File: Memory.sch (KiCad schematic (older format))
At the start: 18 parts, among them U10 74LS05, U11 74HCT00, U12 74LS32, U2 AS6C4008-55PCN, U3 AS6C4008-55PCN, U4 AS6C4008-55PCN, U5 AS6C4008-55PCN, U6 74HCT00, U7 74LS32, U8 74LS32, U9 74LS05

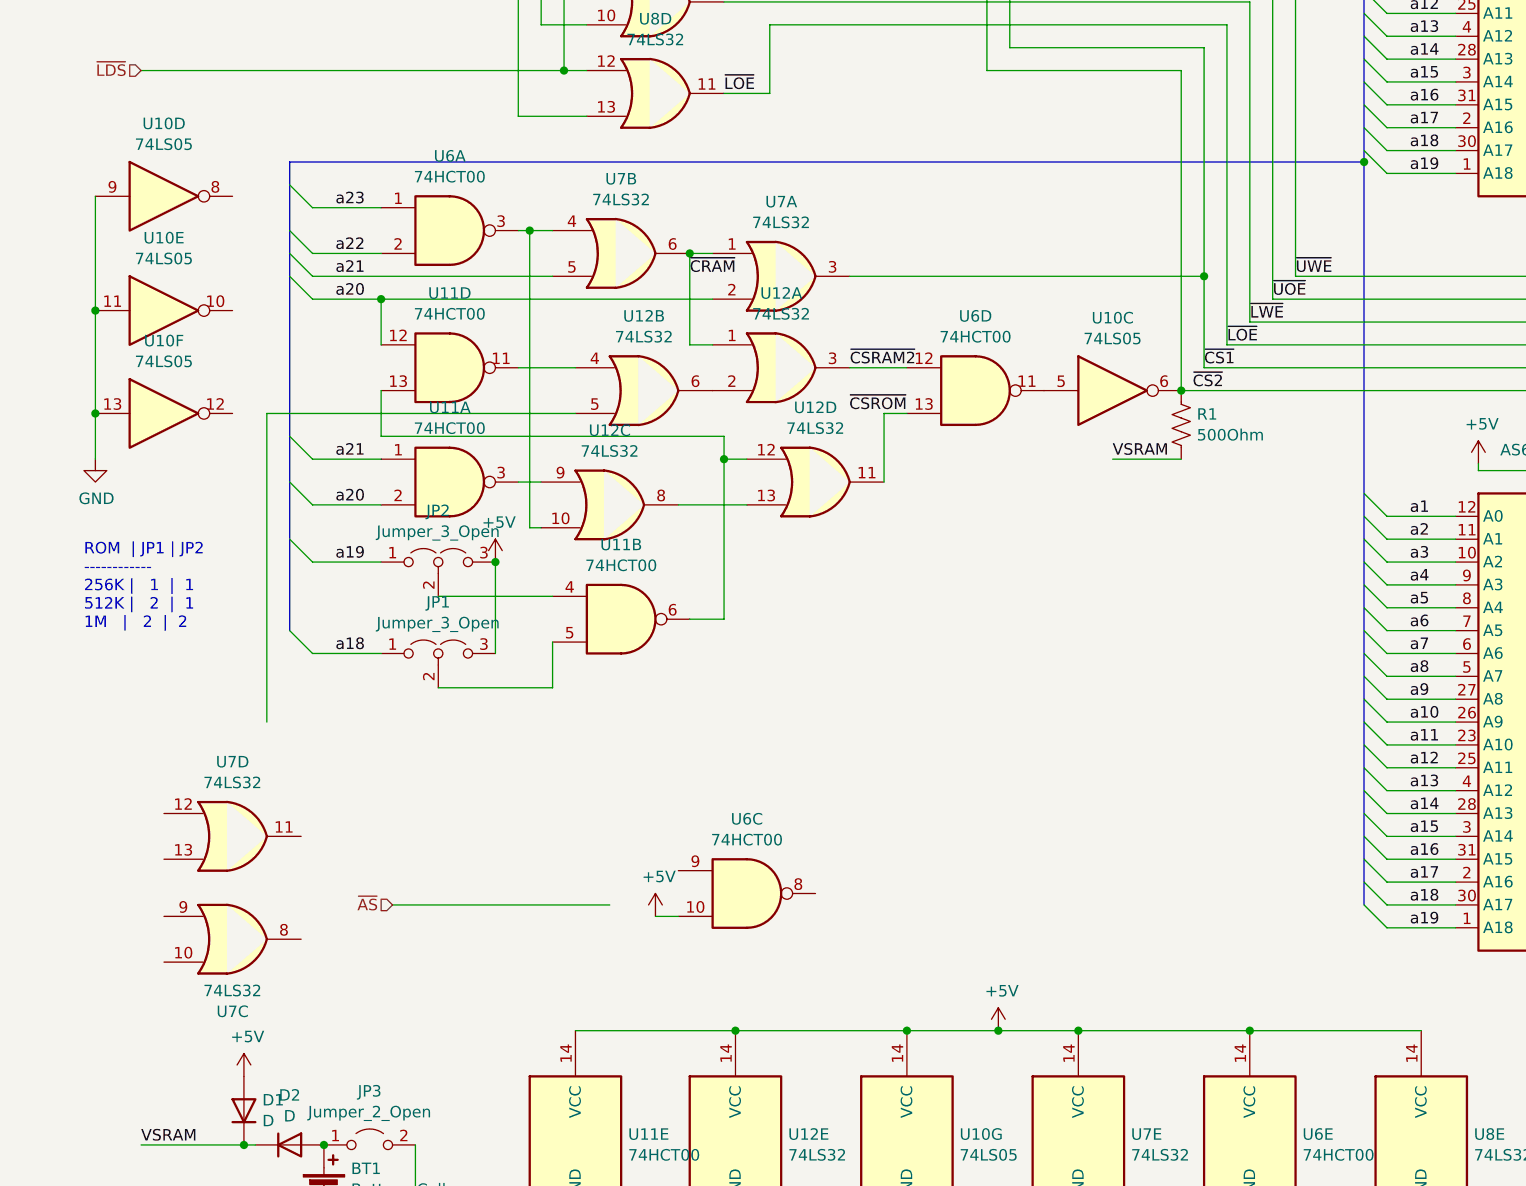
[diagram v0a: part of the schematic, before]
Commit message: rearange
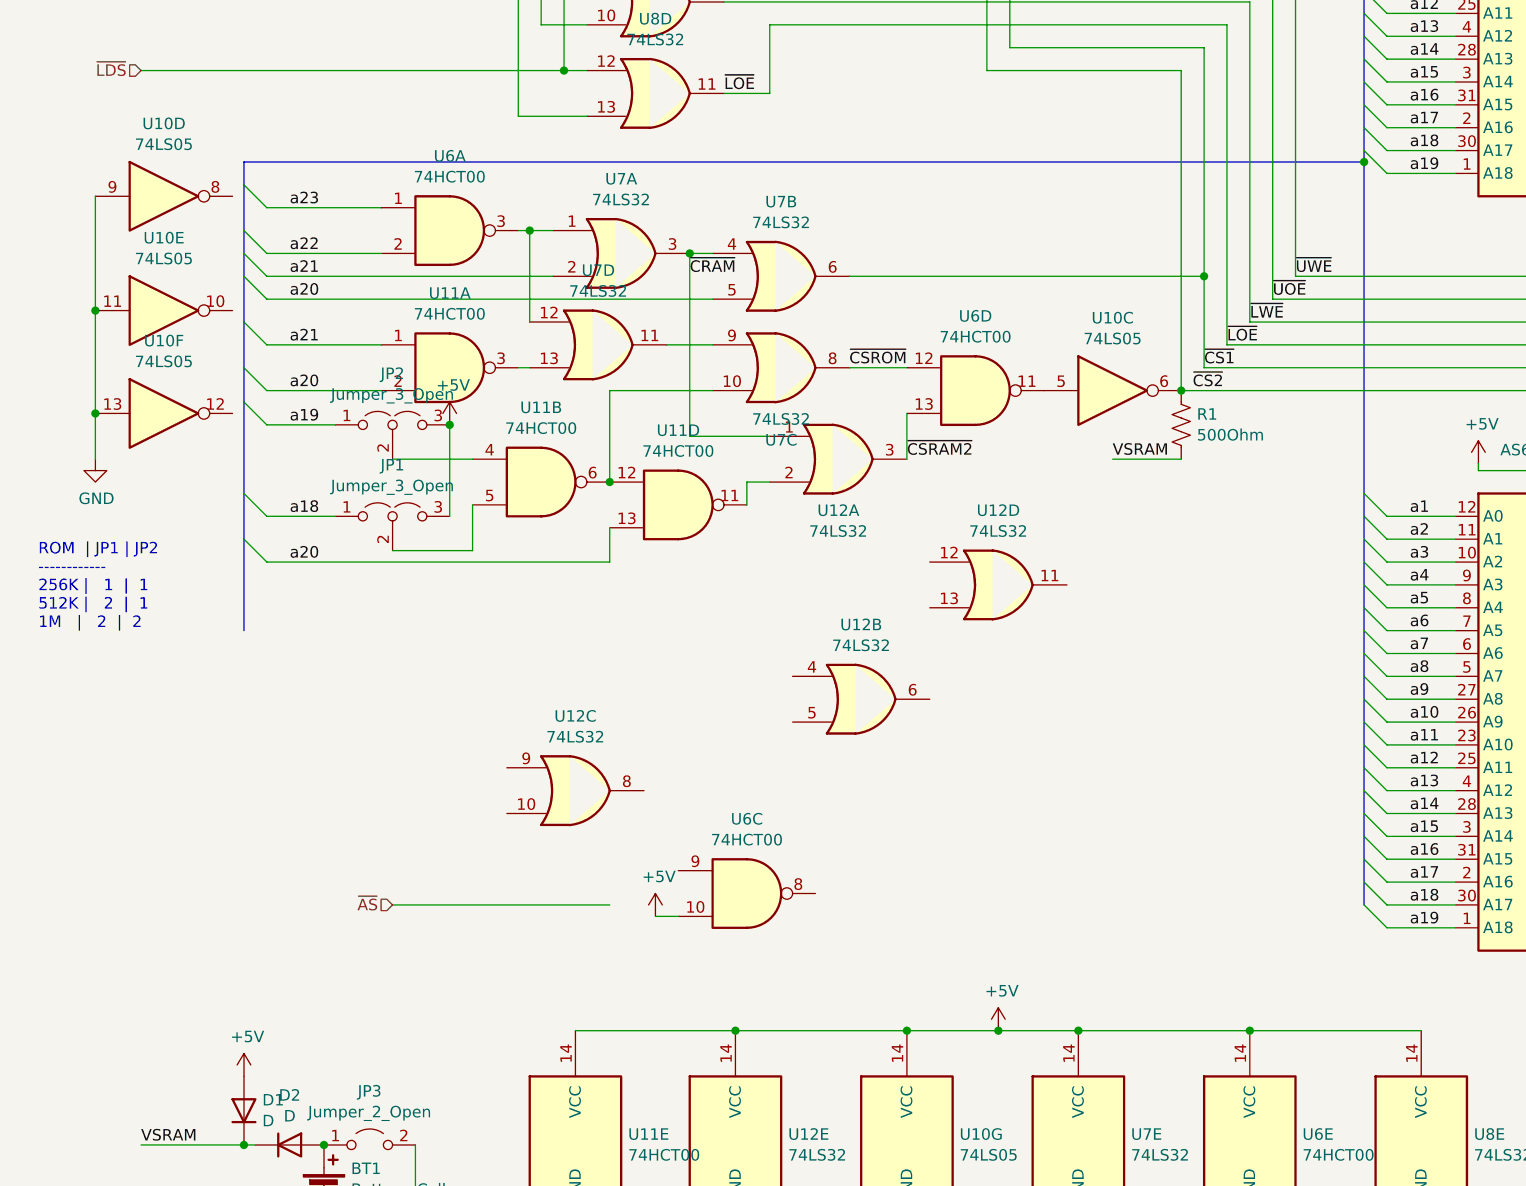
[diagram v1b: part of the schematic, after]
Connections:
- net a20: now also U11.13, U7.5; no longer U11.12, U7.2
- net a21: now also U7.2; no longer U7.5
- net ~CRAM: now also U7.3, U7.4; no longer U7.1, U7.6
- net ~CS1: now also U7.6; no longer U7.3
- net ~CSRAM2: now also U6.13; no longer U6.12
- net ~CSROM: now also U6.12, U7.8; no longer U12.11, U6.13
- net at U7.10: now also U11.12, U11.6
- net at U7.9: now also U7.11
- net at U7.12: now also U6.3, U7.1
- net at U7.13: now also U11.3
- net at U12.4: no longer U11.11
- net at U12.6: no longer U12.2
- net at U12.8: no longer U12.13
- net at U12.9: no longer U11.3
- new net: U11.11, U12.2
- now unconnected: U12.10, U12.12
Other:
- moved on the sheet: JP1, JP2, U11A, U11B, U11D, U12A, U12C, U12D, U7A, U7B, U7C, U7D

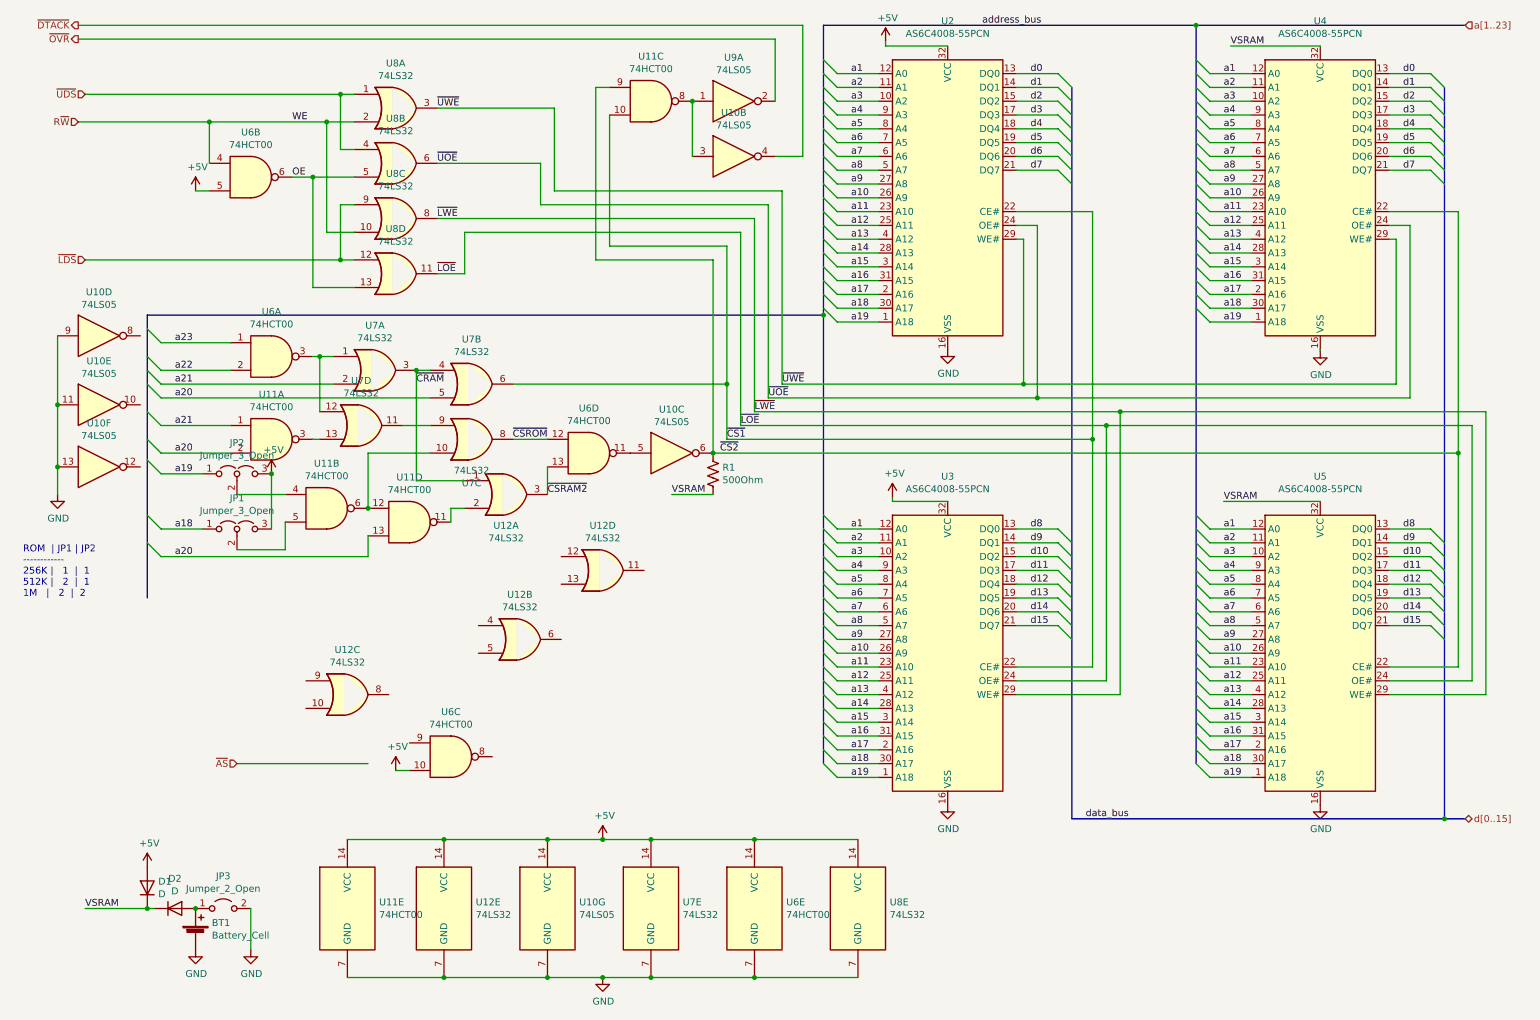
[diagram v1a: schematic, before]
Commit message: more rearange
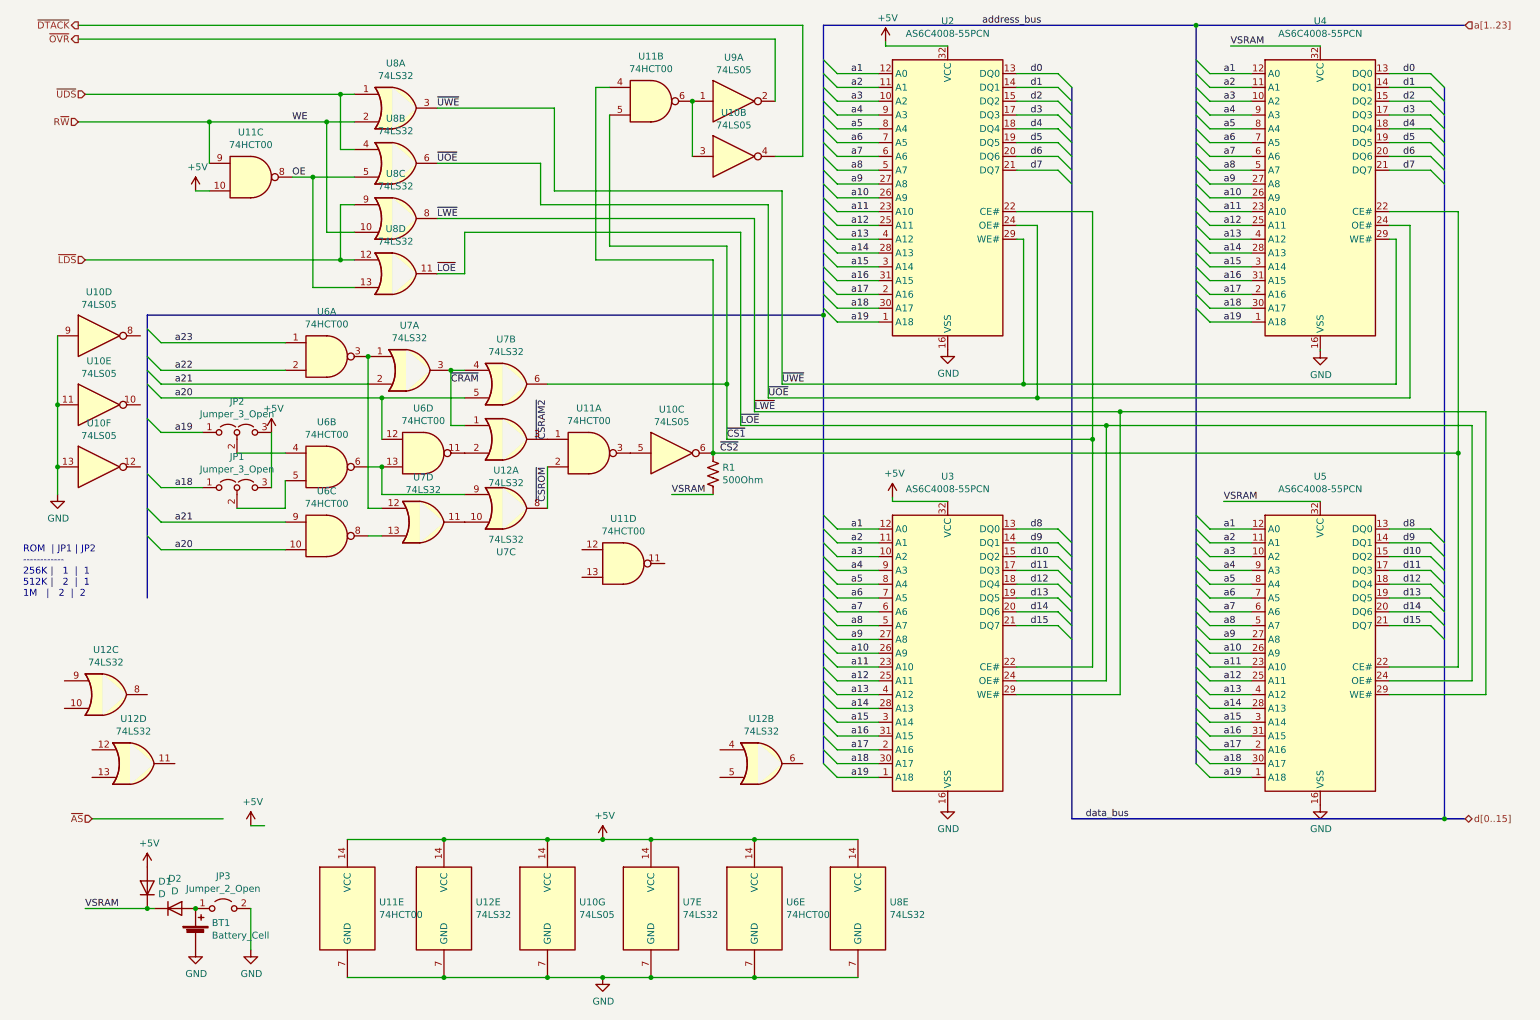
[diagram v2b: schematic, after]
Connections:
- net +5V: now also U11.10; no longer U6.10, U6.5
- net OE: now also U11.8; no longer U6.6
- net R~W: now also U11.9; no longer U6.4
- net a20: now also U6.10, U6.12; no longer U11.13, U11.2
- net a21: now also U6.9; no longer U11.1
- net ~CS1: now also U11.5; no longer U11.10
- net ~CS2: now also U11.4; no longer U11.9
- net ~CSRAM2: now also U11.1; no longer U6.13
- net ~CSROM: now also U11.2; no longer U6.12
- net at JP2.2 (C): now also U6.4; no longer U11.4
- net at JP1.2 (C): now also U6.5; no longer U11.5
- net at U7.11: now also U7.10; no longer U7.9
- net at U7.13: now also U6.8; no longer U11.3
- net at U10.3, U9.1: now also U11.6; no longer U11.8
- net at U10.5: now also U11.3; no longer U6.11
- net at U11.11: no longer U12.2
- new net: U6.13, U6.6, U7.9
- new net: U12.2, U6.11
- now unconnected: U11.12
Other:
- moved on the sheet: JP1, JP2, U11A, U11B, U11C, U11D, U12A, U12B, U12C, U12D, U6A, U6B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
